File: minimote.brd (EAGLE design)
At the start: 160 x 100 mm, 41 parts, among them IC1 ATTINY441/841-SSU, J1 AVR_SPI_PROG_3X2PTH, T1 2N3904

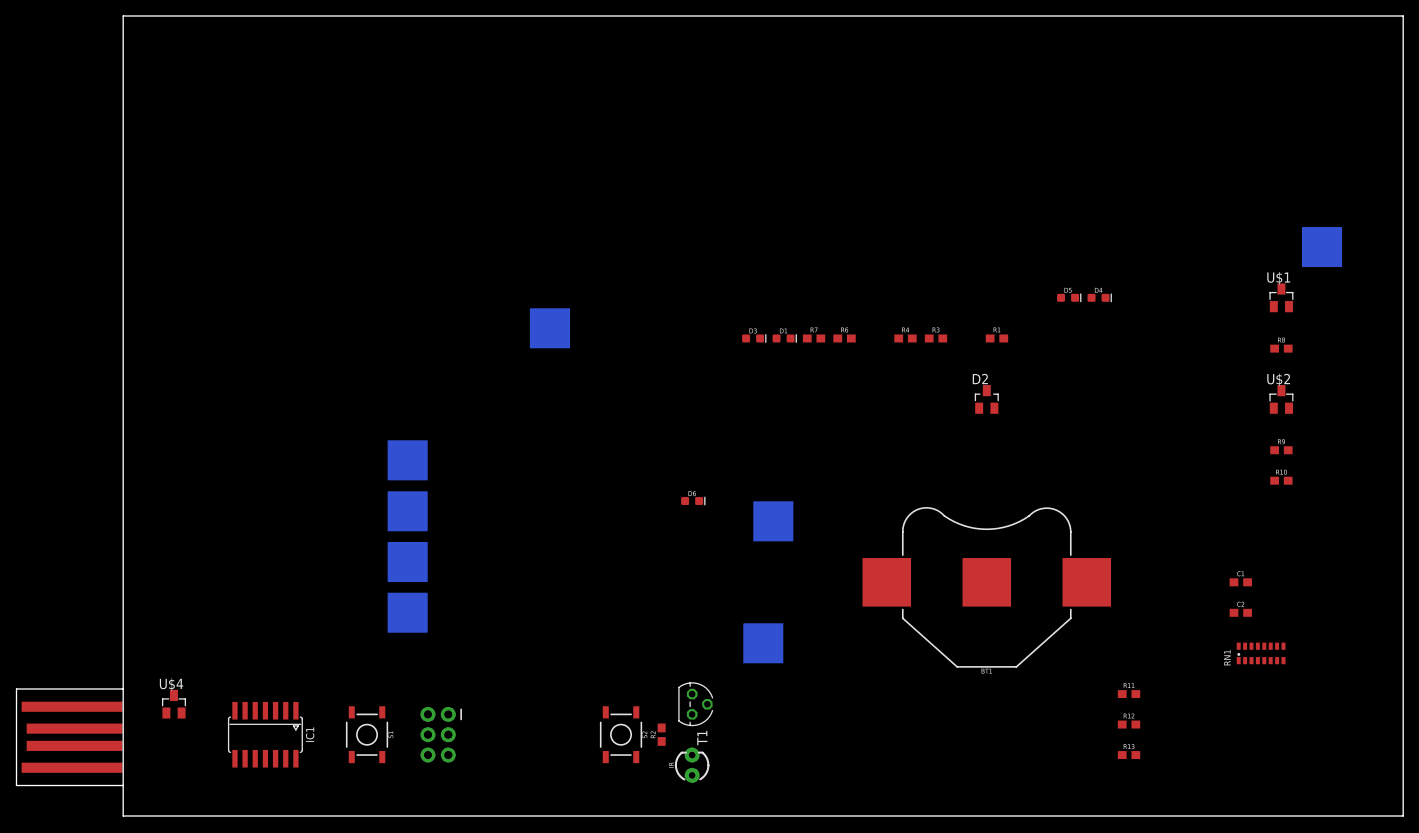
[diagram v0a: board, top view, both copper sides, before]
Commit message: moved parts around
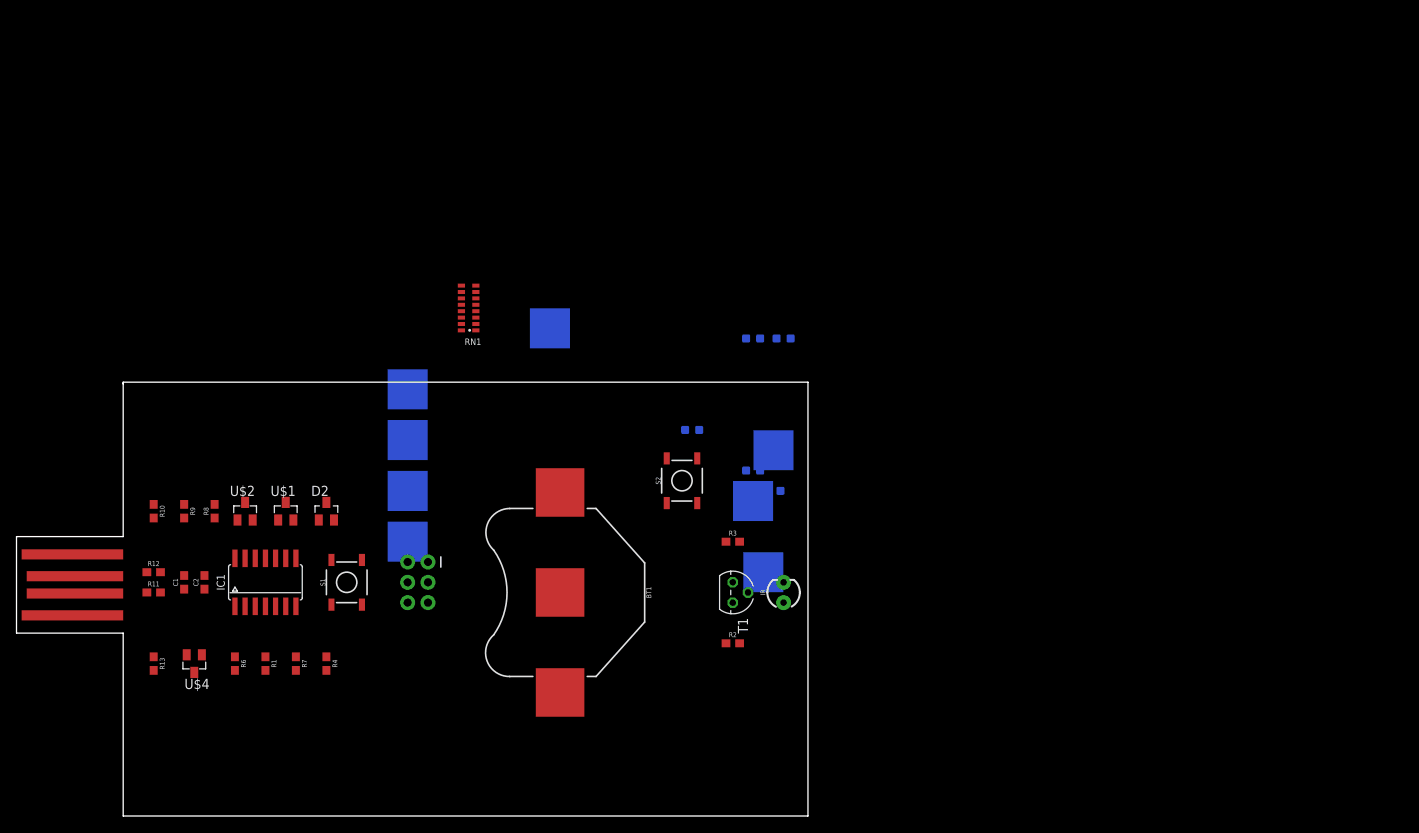
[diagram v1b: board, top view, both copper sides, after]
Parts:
- removed U$3: EDGEUSB, minimote:USBPCB
- added U$13: EDGEUSB, minimote:USBPCB
- moved R10 141.0 mm to (3.81, 38.1), turned to 270 degrees
- moved R9 137.4 mm to (7.62, 38.1), turned to 270 degrees
- moved R8 134.9 mm to (11.4, 38.1), turned to 90 degrees
- moved C1 132.1 mm to (7.62, 29.2), turned to 90 degrees
- moved U$2 130.3 mm to (15.2, 38.1)
- moved C2 129.6 mm to (10.2, 29.2), turned to 90 degrees
- moved U$1 127.3 mm to (20.3, 38.1)
- moved R12 123.4 mm to (3.81, 30.5)
- moved R11 122.6 mm to (3.81, 27.9)
- moved R13 122.5 mm to (3.81, 19.1), turned to 270 degrees
- moved RN1 108.1 mm to (43.2, 63.5), turned to 90 degrees
- moved R1 100.1 mm to (17.8, 19.1), turned to 270 degrees
- moved R6 86.4 mm to (14.0, 19.1), turned to 270 degrees
- moved D2 83.7 mm to (25.4, 38.1)
- moved R4 83.0 mm to (25.4, 19.1), turned to 270 degrees
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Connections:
- new net N$123: D4.C, D5.A, D6.A, R1.2
- new net N$124: D1.C, D3.A, D4.A, D5.C, R4.2
- new net N$125: D1.A, D3.C, D6.C, R7.2
- net GND: now also U$13.GND; no longer U$3.GND
- net LED1: no longer D1.A, D3.C, D6.C, R7.2
- net LED2: no longer D1.C, D3.A, D4.A, D5.C, R4.2
- net LED3: no longer D4.C, D5.A, D6.A, R1.2
- net N$8: now also U$13.DM; no longer U$3.DM
- net N$9: now also U$13.DP; no longer U$3.DP
- net V_USB: now also U$13.VCC; no longer U$3.VCC
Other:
- board size 160 x 100 mm -> 85.6 x 54.2 mm
